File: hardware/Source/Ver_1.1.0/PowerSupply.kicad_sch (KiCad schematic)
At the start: 30 parts, among them J1 Pin Connector, J2 Connector, J3 Connector, SW1 MTS-102-C3, U1 TPS54331DR

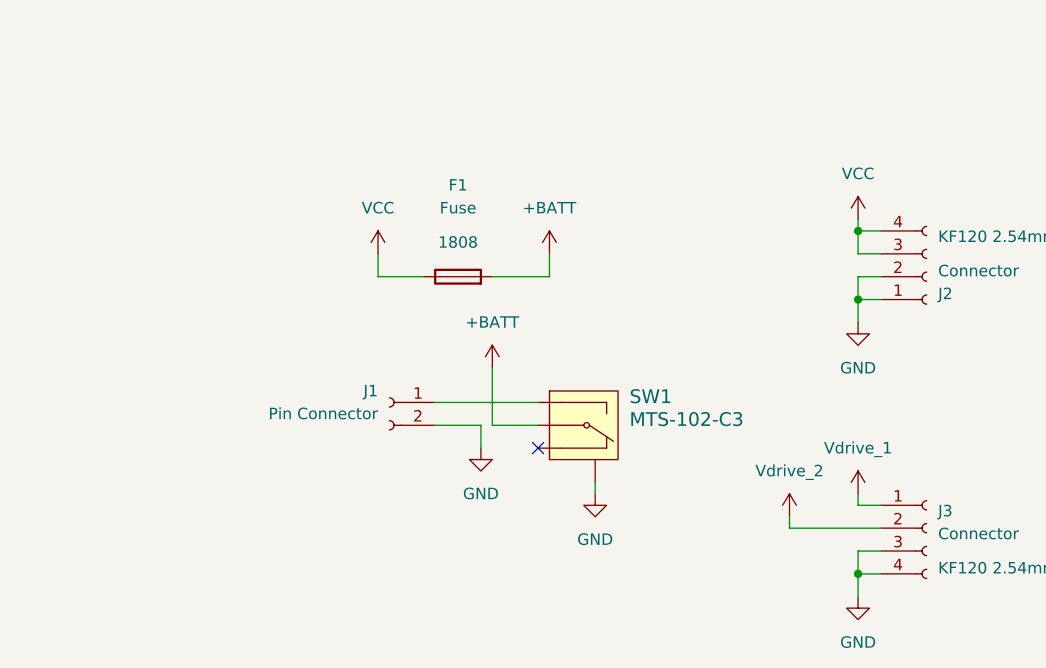
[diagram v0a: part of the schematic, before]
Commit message: Update PCB Ver_1.1.0
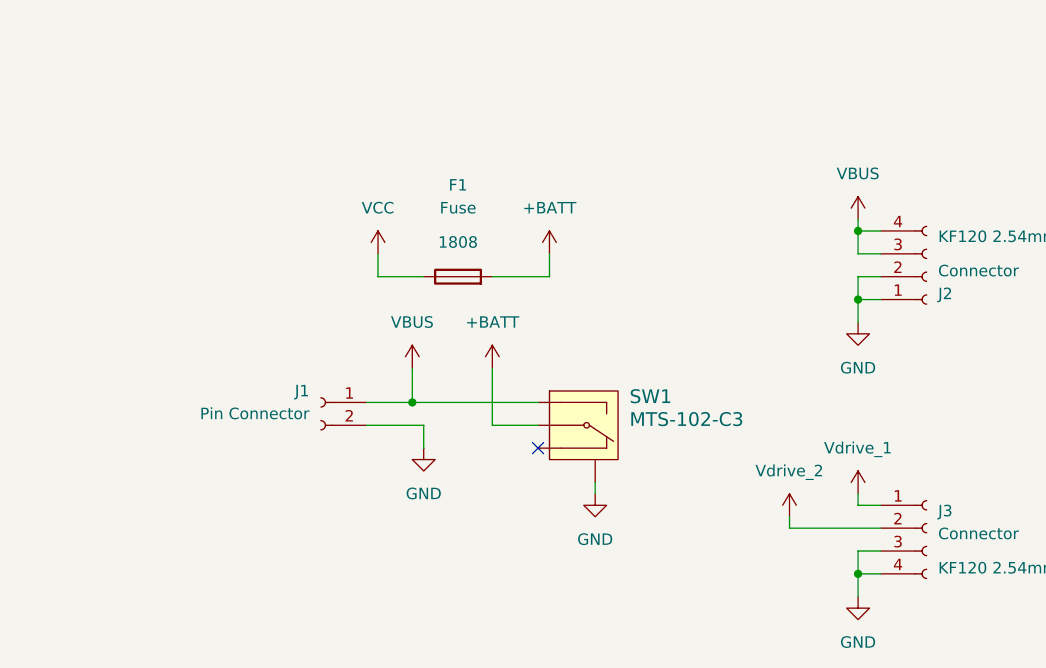
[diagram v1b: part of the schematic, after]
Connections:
- net VCC: no longer J2.3 (Pin_3), J2.4 (Pin_4)
- net VBUS: now reaches J1.1 (Pin_1), SW1.3
- net VBUS: now also J2.3 (Pin_3), J2.4 (Pin_4)
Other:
- moved on the sheet: J1
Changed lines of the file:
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@@
 	)
 	(junction
+		(at 186.69 128.27)
+		(diameter 0)
+		(color 0 0 0 0)
+	)
+	(junction
 		(at 163.83 38.1)
 		(diameter 0)
@@
 	(wire
 		(pts
+			(xy 186.69 128.27) (xy 200.66 128.27)
+		)
+		(stroke
+			(width 0)
+			(type default)
+		)
+	)
+	(wire
+		(pts
 			(xy 236.22 116.84) (xy 236.22 114.3)
 		)
@@
 	(wire
 		(pts
+			(xy 186.69 124.46) (xy 186.69 128.27)
+		)
+		(stroke
+			(width 0)
+			(type default)
+		)
+	)
+	(wire
+		(pts
 			(xy 25.4 30.48) (xy 25.4 33.02)
 		)
@@
 	(wire
 		(pts
-			(xy 194.31 133.35) (xy 194.31 130.81)
+			(xy 187.96 133.35) (xy 187.96 130.81)
 		)
 		(stroke
@@
 	(wire
 		(pts
-			(xy 189.23 128.27) (xy 200.66 128.27)
+			(xy 181.61 128.27) (xy 186.69 128.27)
 		)
 		(stroke
@@
 	(wire
 		(pts
-			(xy 194.31 130.81) (xy 189.23 130.81)
+			(xy 187.96 130.81) (xy 181.61 130.81)
 		)
 		(stroke
@@
 	)
 	(symbol
+		(lib_id "power:VBUS")
+		(at 186.69 124.46 0)
+		(unit 1)
+		(exclude_from_sim no)
+		(in_bom yes)
+		(on_board yes)
+		(dnp no)
+		(fields_autoplaced yes)
+		(property "Reference" "#PWR0186"
+			(at 186.69 128.27 0)
+			(effects
+				(font
+					(size 1.27 1.27)
+				)
+				(hide yes)
+			)
+		)
+		(property "Value" "VBUS"
+			(at 186.69 119.38 0)
+			(effects
+				(font
+					(size 1.27 1.27)
+				)
+			)
+		)
+		(property "Footprint" ""
+			(at 186.69 124.46 0)
+			(effects
+				(font
+					(size 1.27 1.27)
+				)
+				(hide yes)
+			)
+		)
+		(property "Datasheet" ""
+			(at 186.69 124.46 0)
+			(effects
+				(font
+					(size 1.27 1.27)
+				)
+				(hide yes)
+			)
+		)
+		(property "Description" "Power symbol creates a global label with name \"VBUS\""
+			(at 186.69 124.46 0)
+			(effects
+				(font
+					(size 1.27 1.27)
+				)
+				(hide yes)
+			)
+		)
+		(pin "1"
+		)
+		(instances
+			(project "Automative_Hexapod"
+				(path "/c07b6013-2147-4cef-a16e-342deb9ccbf5/e9a15bf3-25b5-4588-8308-b7d586974115"
+					(reference "#PWR0186")
+					(unit 1)
+				)
+			)
+		)
+	)
+	(symbol
 		(lib_id "power:GND")
 		(at 101.6 35.56 270)
@@
 	(symbol
 		(lib_id "automative_hexapod:Pin Connector")
-		(at 184.15 128.27 0)
+		(at 176.53 128.27 0)
 		(mirror y)
 		(unit 1)
@@
 		(dnp no)
 		(property "Reference" "J1"
-			(at 182.88 126.9999 0)
+			(at 175.26 126.9999 0)
 			(effects
 				(font
@@
 		)
 		(property "Value" "Pin Connector"
-			(at 182.88 129.5399 0)
+			(at 175.26 129.5399 0)
 			(effects
 				(font
@@
 		)
 		(property "Footprint" "automative_hexapod:Connector-Pin"
-			(at 183.388 137.16 0)
+			(at 175.768 137.16 0)
 			(effects
 				(font
@@
 		)
 		(property "Datasheet" "~"
-			(at 184.15 128.27 0)
+			(at 176.53 128.27 0)
 			(effects
 				(font
@@
 		)
 		(property "Description" "~"
-			(at 182.118 137.16 0)
+			(at 174.498 137.16 0)
 			(effects
 				(font
@@
 		)
 		(property "Value 2" "~"
-			(at 182.88 131.445 0)
+			(at 175.26 131.445 0)
 			(effects
 				(font
@@
 		)
 		(property "Value 3" "~"
-			(at 182.88 132.715 0)
+			(at 175.26 132.715 0)
 			(effects
 				(font
@@
 		)
 		(property "Value 4" "~"
-			(at 184.15 128.27 0)
+			(at 176.53 128.27 0)
 			(effects
 				(font
@@
 		)
 		(property "Supply Name" "~"
-			(at 182.118 137.16 0)
+			(at 174.498 137.16 0)
 			(effects
 				(font
@@
 		)
 		(property "Supply Part Number" "~"
-			(at 184.15 137.16 0)
+			(at 176.53 137.16 0)
 			(effects
 				(font
@@
 		)
 		(property "Supply URL" "~"
-			(at 184.15 137.16 0)
+			(at 176.53 137.16 0)
 			(effects
 				(font
@@
 	(symbol
 		(lib_id "power:GND")
-		(at 194.31 133.35 0)
+		(at 187.96 133.35 0)
 		(unit 1)
 		(exclude_from_sim no)
@@
 		(fields_autoplaced yes)
 		(property "Reference" "#PWR017"
-			(at 194.31 139.7 0)
+			(at 187.96 139.7 0)
 			(effects
 				(font
@@
 		)
 		(property "Value" "GND"
-			(at 194.31 138.43 0)
+			(at 187.96 138.43 0)
 			(effects
 				(font
@@
 		)
 		(property "Footprint" ""
-			(at 194.31 133.35 0)
+			(at 187.96 133.35 0)
 			(effects
 				(font
@@
 		)
 		(property "Datasheet" ""
-			(at 194.31 133.35 0)
+			(at 187.96 133.35 0)
 			(effects
 				(font
@@
 		)
 		(property "Description" "Power symbol creates a global label with name \"GND\" , ground"
-			(at 194.31 133.35 0)
+			(at 187.96 133.35 0)
 			(effects
 				(font
@@
 	)
 	(symbol
-		(lib_id "power:VCC")
-		(at 236.22 107.95 0)
-		(unit 1)
-		(exclude_from_sim no)
-		(in_bom yes)
-		(on_board yes)
-		(dnp no)
-		(fields_autoplaced yes)
-		(property "Reference" "#PWR022"
-			(at 236.22 111.76 0)
-			(effects
-				(font
-					(size 1.27 1.27)
-				)
-				(hide yes)
-			)
-		)
-		(property "Value" "VCC"
-			(at 236.22 102.87 0)
-			(effects
-				(font
-					(size 1.27 1.27)
-				)
-			)
-		)
-		(property "Footprint" ""
-			(at 236.22 107.95 0)
-			(effects
-				(font
-					(size 1.27 1.27)
-				)
-				(hide yes)
-			)
-		)
-		(property "Datasheet" ""
-			(at 236.22 107.95 0)
-			(effects
-				(font
-					(size 1.27 1.27)
-				)
-				(hide yes)
-			)
-		)
-		(property "Description" "Power symbol creates a global label with name \"VCC\""
-			(at 236.22 107.95 0)
-			(effects
-				(font
-					(size 1.27 1.27)
-				)
-				(hide yes)
-			)
-		)
-		(pin "1"
-		)
-		(instances
-			(project "Automative_Hexapod"
-				(path "/c07b6013-2147-4cef-a16e-342deb9ccbf5/e9a15bf3-25b5-4588-8308-b7d586974115"
-					(reference "#PWR022")
-					(unit 1)
-				)
-			)
-		)
-	)
-	(symbol
 		(lib_id "automative_hexapod:Fuse_1808")
 		(at 191.77 114.3 0)
@@
 					(unit 1)
 				)
+			)
+		)
+	)
+	(symbol
+		(lib_id "power:VBUS")
+		(at 236.22 107.95 0)
+		(unit 1)
+		(exclude_from_sim no)
+		(in_bom yes)
+		(on_board yes)
+		(dnp no)
+		(fields_autoplaced yes)
+		(property "Reference" "#PWR0187"
+			(at 236.22 111.76 0)
+			(effects
+				(font
+					(size 1.27 1.27)
+				)
+				(hide yes)
+			)
+		)
+		(property "Value" "VBUS"
+			(at 236.22 102.87 0)
+			(effects
+				(font
+					(size 1.27 1.27)
+				)
+			)
+		)
+		(property "Footprint" ""
+			(at 236.22 107.95 0)
+			(effects
+				(font
+					(size 1.27 1.27)
+				)
+				(hide yes)
+			)
+		)
+		(property "Datasheet" ""
+			(at 236.22 107.95 0)
+			(effects
+				(font
+					(size 1.27 1.27)
+				)
+				(hide yes)
+			)
+		)
+		(property "Description" "Power symbol creates a global label with name \"VBUS\""
+			(at 236.22 107.95 0)
+			(effects
+				(font
+					(size 1.27 1.27)
+				)
+				(hide yes)
+			)
+		)
+		(pin "1"
+		)
+		(instances
+			(project "Automative_Hexapod"
+				(path "/c07b6013-2147-4cef-a16e-342deb9ccbf5/e9a15bf3-25b5-4588-8308-b7d586974115"
+					(reference "#PWR0187")
+					(unit 1)
+				)
